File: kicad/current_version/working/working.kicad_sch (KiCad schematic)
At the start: 1 part, among them J1 scuath

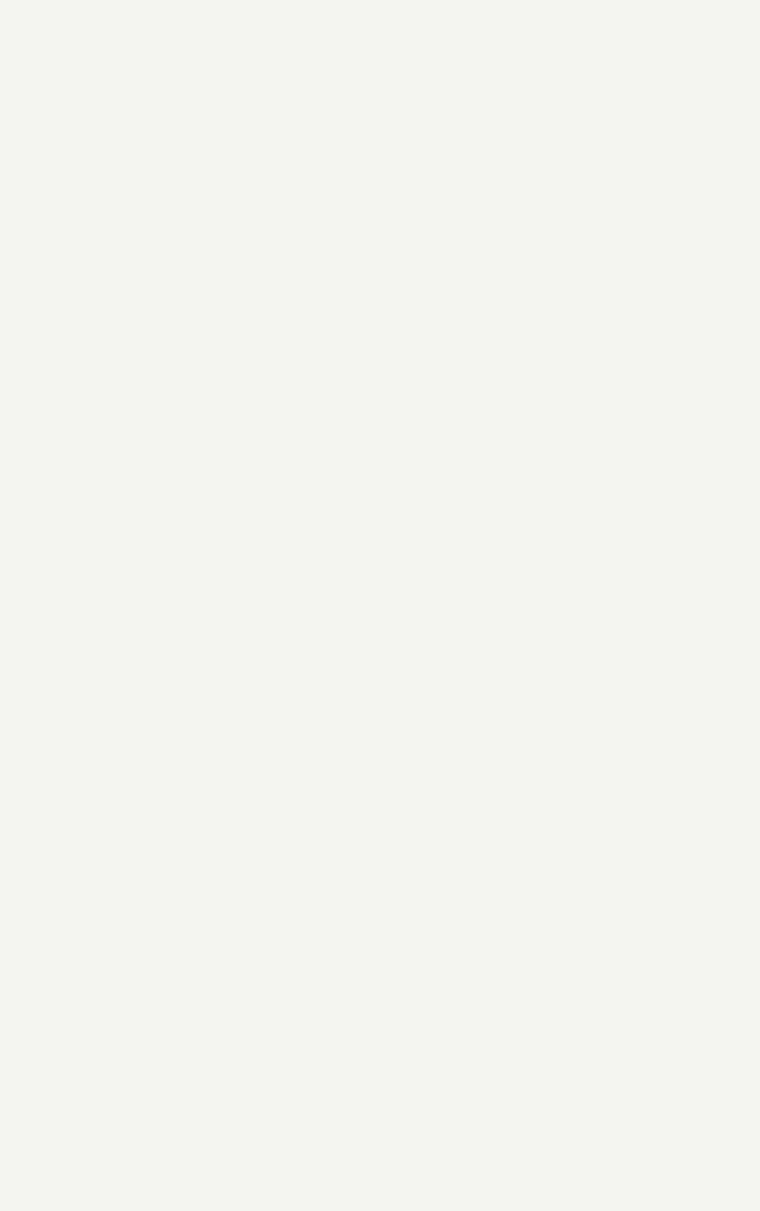
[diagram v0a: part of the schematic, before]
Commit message: commiting after auto generation
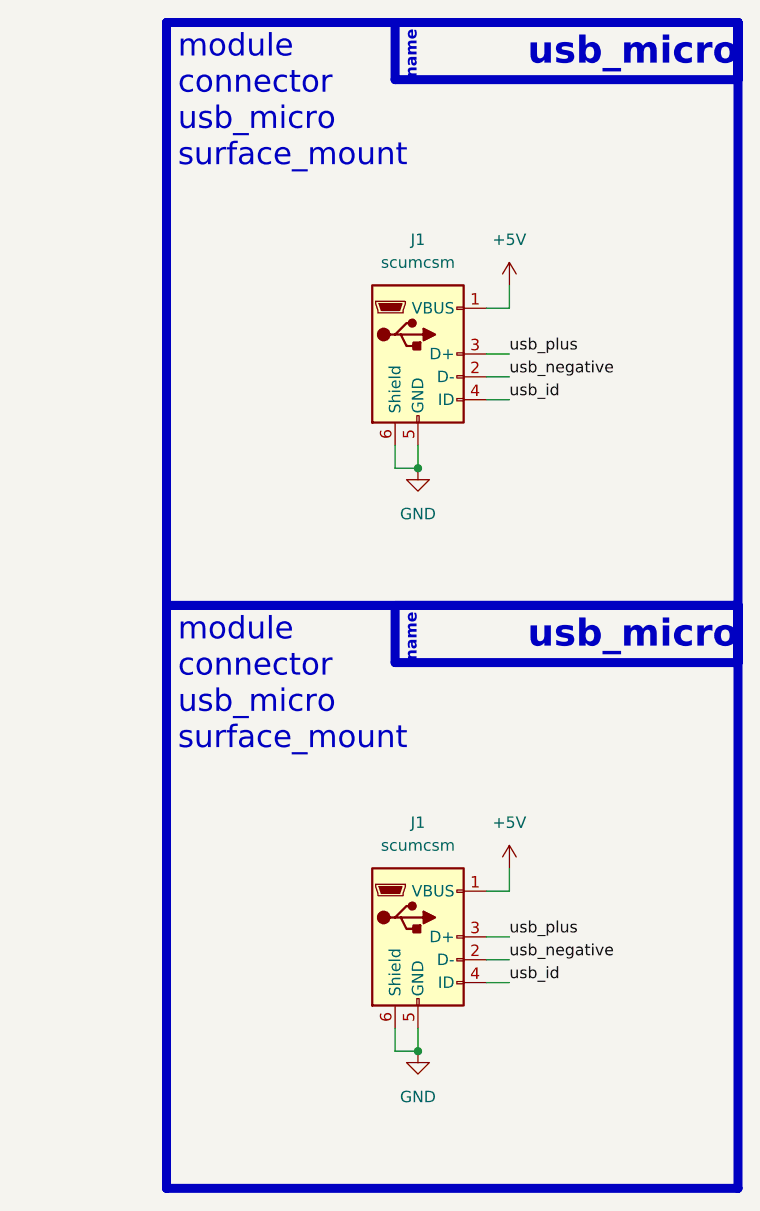
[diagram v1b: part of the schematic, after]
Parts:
- added J1 (x2): scumcsm, oomlout_oomp_part_footprints:scumcsm_electronic_socket_usb_micro_surface_mount, symbol oomlout_oomp_part_symbols:scumcsm_electronic_socket_usb_micro_surface_mount
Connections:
- net +5V: now also J1.1 (VBUS), J1.1 (VBUS)
- net GND: now also J1.5 (GND), J1.5 (GND), J1.6 (Shield), J1.6 (Shield)
- net usb_negative: now also J1.2 (D-), J1.2 (D-)
- net usb_plus: now also J1.3 (D+), J1.3 (D+)
- new net usb_id: J1.4 (ID), J1.4 (ID)
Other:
- note added: "module connector usb_micro surface_mount"
- note added: "usb_micro"
